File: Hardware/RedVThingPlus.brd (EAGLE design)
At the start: 58.4 x 22.9 mm, 139 parts, among them J1 FEMALE 2x3, J2 USB Female Type C Connector, J4 QWIIC_RIGHT_ANGLE, Q1 3.1A/30V/105mΩ, U1 MCP73831, U2 AP2127K-1.8V, U3 AP2112-3.3V, U4 MK22FN128VLH10, U5 32MBit, U6 FE310, Y1 32.768KHZ, Y2 16MHz

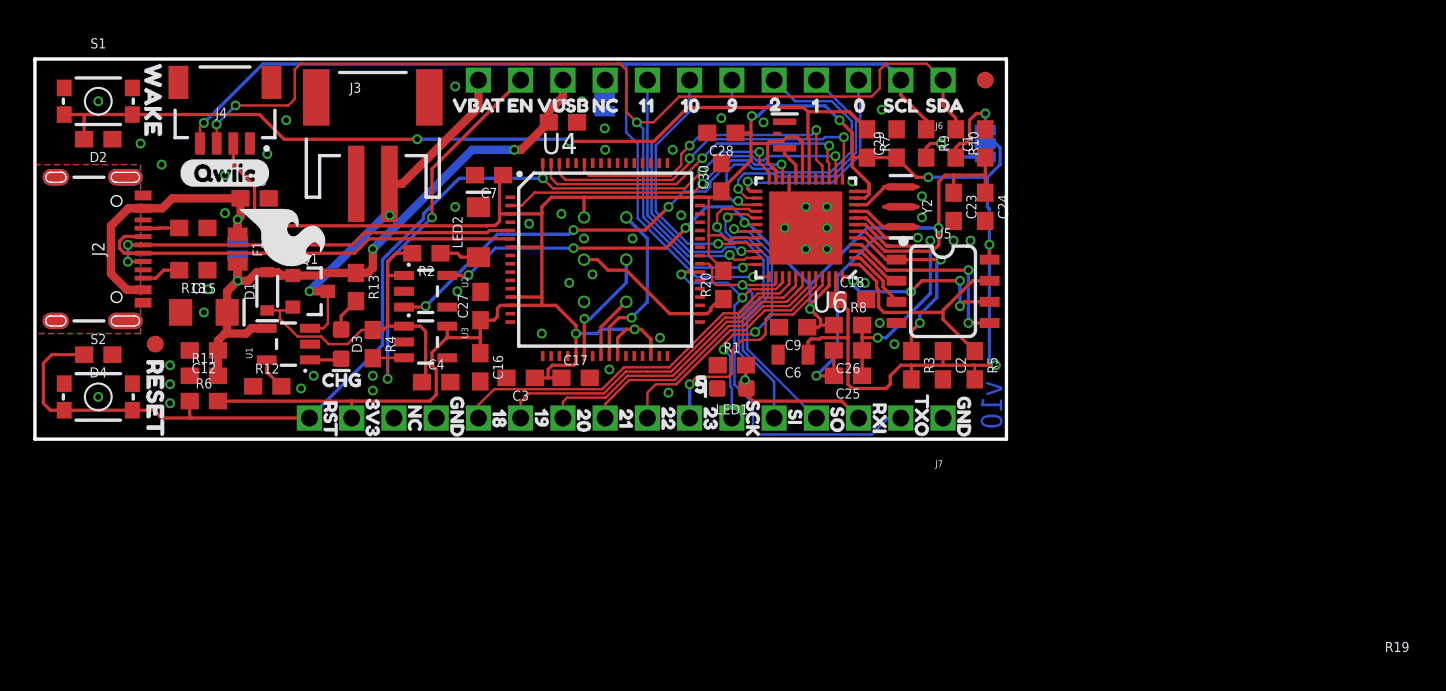
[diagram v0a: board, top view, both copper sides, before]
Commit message: post qc double check changes
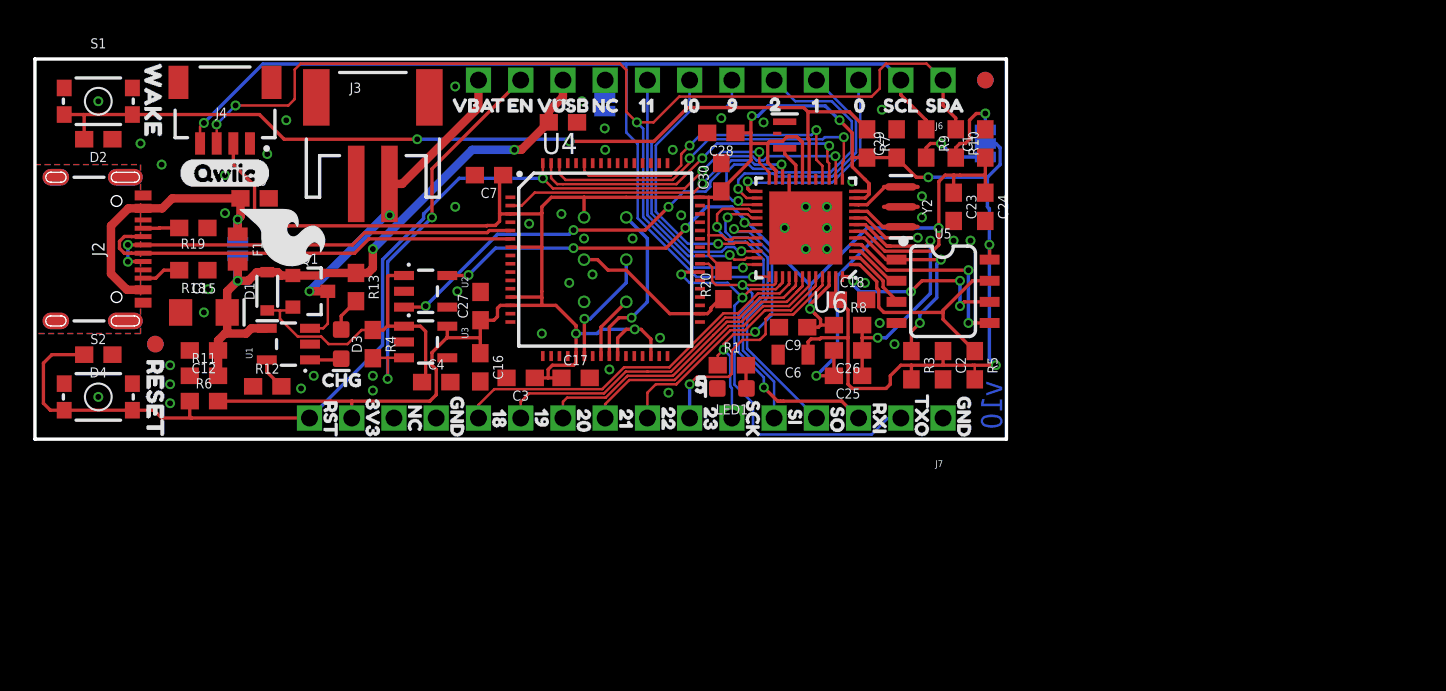
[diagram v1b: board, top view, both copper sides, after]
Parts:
- removed LED2: RED, SparkFun-LED:LED-1206
- removed R2: 10k, SparkFun-Resistors:0603
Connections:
- removed net N$2: LED2.A, R2.1
- net 5V: no longer R2.2
- net GND: no longer LED2.C
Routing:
- net 5V: track 21.8 -> 19.2 mm
- net N$2: track 2.37 -> 0.00 mm
- net RXI: track 21.4 -> 19.9 mm
- net SPI_SCK: track 16.3 -> 17.4 mm
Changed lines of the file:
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@@
 <layer number="23" name="tOrigins" color="15" fill="1" visible="yes" active="yes"/>
 <layer number="24" name="bOrigins" color="15" fill="1" visible="yes" active="yes"/>
-<layer number="25" name="tNames" color="7" fill="1" visible="no" active="yes"/>
+<layer number="25" name="tNames" color="7" fill="1" visible="yes" active="yes"/>
 <layer number="26" name="bNames" color="7" fill="1" visible="no" active="yes"/>
-<layer number="27" name="tValues" color="7" fill="1" visible="no" active="yes"/>
+<layer number="27" name="tValues" color="7" fill="1" visible="yes" active="yes"/>
 <layer number="28" name="bValues" color="7" fill="1" visible="no" active="yes"/>
 <layer number="29" name="tStop" color="2" fill="3" visible="yes" active="yes"/>
@@
 <attribute name="VALUE" x="41.91" y="3.683" size="0.6096" layer="27" font="vector" ratio="20" align="top-center"/>
 </element>
-<element name="R2" library="SparkFun-Resistors" package="0603" value="10k" x="23.542" y="11.176" smashed="yes" rot="R180">
-<attribute name="NAME" x="23.542" y="10.414" size="0.6096" layer="25" font="vector" ratio="20" rot="R180" align="bottom-center"/>
-<attribute name="PROD_ID" value="RES-00824" x="23.542" y="11.176" size="1.778" layer="27" rot="R180" display="off"/>
-<attribute name="VALUE" x="23.542" y="11.938" size="0.6096" layer="27" font="vector" ratio="20" rot="R180" align="top-center"/>
-</element>
 <element name="C10" library="SparkFun-Capacitors" package="0603" value="0.1uF" x="13.208" y="14.478" smashed="yes">
 <attribute name="NAME" x="13.208" y="15.24" size="0.6096" layer="25" font="vector" ratio="20" align="bottom-center"/>
@@
 <attribute name="VALUE" x="10.16" y="6.477" size="0.6096" layer="27" font="vector" ratio="20" align="top-center"/>
 </element>
-<element name="LED2" library="SparkFun-LED" package="LED-1206" value="RED" x="26.67" y="12.446" smashed="yes" rot="R90">
-<attribute name="NAME" x="25.7175" y="12.446" size="0.6096" layer="25" font="vector" ratio="20" rot="R90" align="bottom-center"/>
-<attribute name="PROD_ID" value="DIO-09912" x="26.67" y="12.446" size="1.778" layer="27" rot="R90" display="off"/>
-<attribute name="VALUE" value="RED" x="27.6225" y="12.446" size="0.6096" layer="27" font="vector" ratio="20" rot="R90" align="top-center"/>
-</element>
 <element name="LED1" library="SparkFun-LED" package="LED-0603" value="BLUE" x="41.91" y="3.048" smashed="yes" rot="R180">
 <attribute name="NAME" x="41.91" y="2.0955" size="0.6096" layer="25" font="vector" ratio="20" rot="R180" align="bottom-center"/>
@@
 </element>
 <element name="R19" library="SparkFun-Resistors" package="0603" value="5.1k" x="9.525" y="12.7" smashed="yes" rot="R180">
-<attribute name="NAME" x="81.915" y="-12.192" size="0.6096" layer="25" font="vector" ratio="20" rot="R180" align="bottom-center"/>
+<attribute name="NAME" x="9.5035" y="12.0635" size="0.6096" layer="25" font="vector" ratio="20" rot="R180" align="bottom-center"/>
 <attribute name="PROD_ID" value="RES-12083" x="9.525" y="12.7" size="1.778" layer="27" rot="R180" display="off"/>
 <attribute name="VALUE" x="9.525" y="13.462" size="0.6096" layer="27" font="vector" ratio="20" rot="R180" align="top-center"/>
@@
 <signal name="5V">
 <contactref element="U2" pad="1"/>
-<contactref element="R2" pad="2"/>
 <contactref element="U3" pad="1"/>
 <contactref element="R4" pad="1"/>
@@
 <wire x1="23.495" y1="3.644" x2="23.495" y2="6.477" width="0.2032" layer="1"/>
 <wire x1="23.495" y1="6.477" x2="23.18" y2="6.792" width="0.2032" layer="1"/>
-<wire x1="21.717" y1="11.176" x2="22.692" y2="11.176" width="0.2032" layer="1"/>
 <wire x1="21.209" y1="6.792" x2="21.209" y2="9.779" width="0.2032" layer="1"/>
-<wire x1="21.209" y1="9.779" x2="21.209" y2="10.668" width="0.2032" layer="1"/>
-<wire x1="21.209" y1="10.668" x2="21.717" y2="11.176" width="0.2032" layer="1"/>
 <wire x1="22.1949" y1="9.84" x2="21.27" y2="9.84" width="0.2032" layer="1"/>
 <wire x1="21.27" y1="9.84" x2="21.209" y2="9.779" width="0.2032" layer="1"/>
 </signal>
 <signal name="GND">
-<contactref element="LED2" pad="C"/>
 <contactref element="LED1" pad="C"/>
 <contactref element="C16" pad="2"/>
@@
 <wire x1="57.277" y1="13.97" x2="57.277" y2="15.748" width="0.2032" layer="16"/>
 </signal>
-<signal name="N$2">
-<contactref element="R2" pad="1"/>
-<contactref element="LED2" pad="A"/>
-<wire x1="26.67" y1="10.946" x2="25.63" y2="10.946" width="0.2032" layer="1"/>
-<wire x1="25.4" y1="11.176" x2="24.392" y2="11.176" width="0.2032" layer="1"/>
-<wire x1="25.63" y1="10.946" x2="25.4" y2="11.176" width="0.2032" layer="1"/>
-</signal>
 <signal name="VUSB">
 <contactref element="F1" pad="1"/>
@@
 <wire x1="46.99" y1="18.5843" x2="46.6937" y2="18.288" width="0.1524" layer="16"/>
 <wire x1="46.99" y1="16.8002" x2="47.355" y2="16.4352" width="0.1524" layer="1"/>
-<wire x1="46.99" y1="17.5542" x2="46.99" y2="17.5542" width="0.1524" layer="1"/>
 <wire x1="46.99" y1="16.8002" x2="46.99" y2="18.5843" width="0.1524" layer="1"/>
 <via x="46.99" y="18.5843" extent="1-16" drill="0.35"/>
@@
 <contactref element="J7" pad="3"/>
 <wire x1="40.95055" y1="9.271" x2="40.7242" y2="9.49735" width="0.1524" layer="1"/>
-<wire x1="44.45" y1="9.271" x2="44.555" y2="9.376" width="0.1524" layer="1"/>
 <wire x1="42.545" y1="9.271" x2="44.45" y2="9.271" width="0.1524" layer="1"/>
 <wire x1="49.53" y1="1.27" x2="48.514" y2="2.286" width="0.2032" layer="1"/>
-<via x="42.7002" y="3.556" extent="1-16" drill="0.35"/>
-<wire x1="42.672" y1="7.84576875" x2="42.813115625" y2="7.986884375" width="0.1524" layer="16"/>
-<wire x1="42.813115625" y1="7.986884375" x2="43.130615625" y2="8.304384375" width="0.1524" layer="16"/>
+<via x="43.8327" y="3.112" extent="1-16" drill="0.35"/>
 <wire x1="43.130615625" y1="8.304384375" x2="43.130615625" y2="8.763" width="0.1524" layer="16"/>
 <via x="42.545" y="9.271" extent="1-16" drill="0.35"/>
@@
 <wire x1="43.130615625" y1="8.763" x2="42.622615625" y2="9.271" width="0.1524" layer="16"/>
 <wire x1="42.622615625" y1="9.271" x2="42.545" y2="9.271" width="0.1524" layer="16"/>
-<wire x1="42.813115625" y1="7.986884375" x2="42.672" y2="7.84576875" width="0.1524" layer="16"/>
-<wire x1="42.672" y1="7.84576875" x2="42.3192" y2="7.49296875" width="0.1524" layer="16"/>
+<wire x1="43.130615625" y1="8.304384375" x2="42.3192" y2="7.49296875" width="0.1524" layer="16"/>
 <wire x1="42.3192" y1="7.49296875" x2="42.3192" y2="5.222375" width="0.1524" layer="16"/>
 <contactref element="U6" pad="38"/>
@@
 <wire x1="44.555" y1="9.376" x2="44.555" y2="9.775" width="0.1524" layer="1"/>
 <wire x1="40.7242" y1="9.49735" x2="40.7242" y2="10.3298" width="0.1524" layer="1"/>
-<wire x1="40.7242" y1="10.3298" x2="40.509" y2="10.545" width="0.1524" layer="1"/>
 <contactref element="U4" pad="40"/>
 <wire x1="40.7242" y1="10.3298" x2="40.509" y2="10.545" width="0.1524" layer="1"/>
 <wire x1="40.509" y1="10.545" x2="39.99" y2="10.545" width="0.1524" layer="1"/>
-<wire x1="42.7002" y1="4.841375" x2="42.7002" y2="3.556" width="0.1524" layer="16"/>
-<wire x1="42.3192" y1="5.222375" x2="42.7002" y2="4.841375" width="0.1524" layer="16"/>
-<wire x1="48.514" y1="2.286" x2="43.18" y2="2.286" width="0.2032" layer="1"/>
-<wire x1="42.7002" y1="2.7658" x2="42.7002" y2="3.556" width="0.2032" layer="1"/>
-<wire x1="43.18" y1="2.286" x2="42.7002" y2="2.7658" width="0.2032" layer="1"/>
+<wire x1="43.8327" y1="3.708875" x2="43.8327" y2="3.112" width="0.1524" layer="16"/>
+<wire x1="42.3192" y1="5.222375" x2="43.8327" y2="3.708875" width="0.1524" layer="16"/>
+<wire x1="48.514" y1="2.286" x2="45" y2="2.286" width="0.2032" layer="1"/>
+<wire x1="45" y1="2.286" x2="44.8327" y2="2.286" width="0.2032" layer="1"/>
+<wire x1="44.8327" y1="2.286" x2="44.6587" y2="2.286" width="0.2032" layer="1"/>
+<wire x1="44.6587" y1="2.286" x2="43.8327" y2="3.112" width="0.2032" layer="1"/>
 </signal>
 <signal name="TXO">
@@
 <wire x1="42" y1="6.2962" x2="41.41364375" y2="5.70984375" width="0.1524" layer="1"/>
 <wire x1="41.41364375" y1="5.70984375" x2="41.41364375" y2="5.3858" width="0.1524" layer="1"/>
-<wire x1="41.8112" y1="4.98824375" x2="41.06" y2="4.445" width="0" layer="19" extent="1-16"/>
+<wire x1="41.41364375" y1="5.3858" x2="41.06" y2="5.03215625" width="0.1524" layer="1"/>
+<wire x1="41.06" y1="5.03215625" x2="41.06" y2="4.445" width="0.1524" layer="1"/>
 </signal>
 <signal name="IO10">
@@
 <contactref element="I2C" pad="3"/>
 <wire x1="55.372" y1="16.93" x2="55.372" y2="17.526" width="0.2032" layer="1"/>
-<wire x1="57.15" y1="18.5928" x2="57.1274" y2="18.5928" width="0.2032" layer="16"/>
 <wire x1="55.372" y1="17.526" x2="55.626" y2="17.78" width="0.2032" layer="1"/>
 <wire x1="55.9435" y1="17.78" x2="56.1975" y2="18.034" width="0.2032" layer="1"/>
